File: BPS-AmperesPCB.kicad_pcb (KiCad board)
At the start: 2 copper layers, 70 x 58 mm, 42 parts, among them J1 Conn_01x04, J2 PeripheralCANConnector, J3 PeripheralCANConnector, U1 PeripheralSOM, U2 INA145UA/2K5, U3 AMC1300BDWV, U4 RO-123.3S_HP

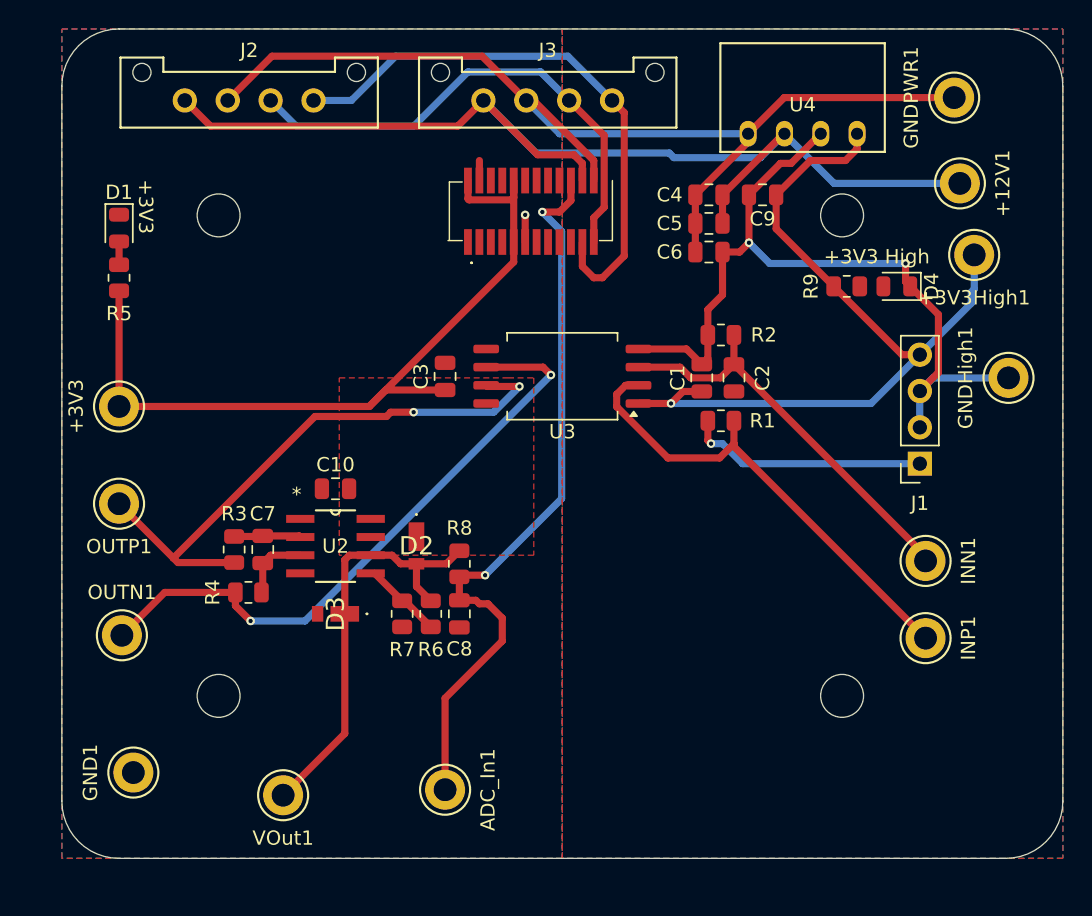
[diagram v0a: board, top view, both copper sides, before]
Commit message: reviewable part 2
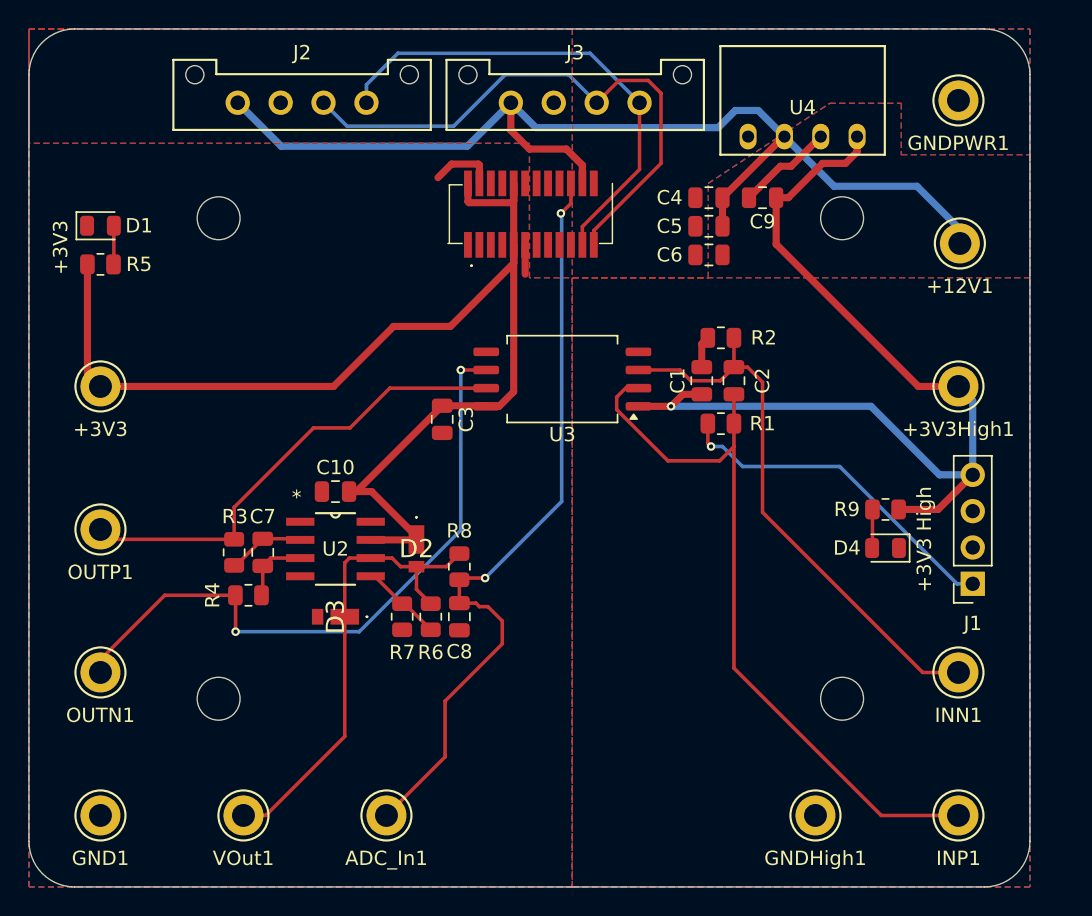
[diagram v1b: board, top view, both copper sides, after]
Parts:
- moved GNDHigh1 33.4 mm to (123.5, 88.6), turned to 0 degrees
- moved D4 18.3 mm to (128.4, 69.9)
- moved R9 15.8 mm to (128.4, 67.2), turned to 180 degrees
- moved INP1 12.6 mm to (133.5, 88.6), turned to 180 degrees
- moved +3V3High1 9.27 mm to (133.5, 58.6)
- moved J1 9.18 mm to (134.5, 72.4)
- moved INN1 8.13 mm to (133.5, 78.6), turned to 180 degrees
- moved ADC_In1 4.48 mm to (93.5, 88.6), turned to 0 degrees
- moved +12V1 4.20 mm to (133.6, 48.6), turned to 0 degrees
- moved GND1 3.78 mm to (73.5, 88.6), turned to 180 degrees
- moved J2 3.70 mm to (83.1, 38.8)
- moved VOut1 3.11 mm to (83.5, 88.6)
- moved C3 3.01 mm to (97.4, 60.9), turned to -90 degrees
- moved OUTN1 3.00 mm to (73.5, 78.6), turned to 180 degrees
- moved OUTP1 2.22 mm to (73.5, 68.6)
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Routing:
- net GNDPWR: track 73.0 -> 0.00 mm
- net GND High: track 56.7 -> 9.02 mm, vias 2 -> 0
- net +3V3: track 57.1 -> 86.9 mm
- net /INP: track 33.5 -> 51.9 mm
- net +3V3 High: track 56.3 -> 68.8 mm
- net /INN: track 28.7 -> 39.3 mm
- net /OUTP: track 41.3 -> 33.0 mm, vias 2 -> 0
- net Net-(J1-Pin_1): track 16.9 -> 24.0 mm
- net Net-(J2-CAN_L): track 40.3 -> 34.3 mm
- net Net-(J2-CAN_H): track 35.2 -> 40.1 mm
- net GND: track 3.30 -> 6.65 mm, vias 1 -> 0
- net Net-(D2-A): track 30.0 -> 33.3 mm
- net Net-(D4-A): track 0.00 -> 2.71 mm
- net /OUTN: track 44.5 -> 46.4 mm
- net +12V: track 77.5 -> 76.0 mm
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- added copper zone on B.Cu, net GND High
- added copper zone on F.Cu, net GND High
- added copper zone on B.Cu, net GNDPWR
- added copper zone on F.Cu, net GNDPWR
- removed copper zone on F.Cu, net +3V3
- removed copper zone on B.Cu, net /MISO
- removed copper zone on F.Cu, net /MISO
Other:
- board size 70 x 58 mm -> 70 x 60 mm
